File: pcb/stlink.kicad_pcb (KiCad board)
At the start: 4 copper layers, 36.5 x 20 mm, 41 parts, among them J1 USB_A, Q1 S9013, U1 XC6206P332MR, U2 GD32F103CBT6, Y1 8MHz

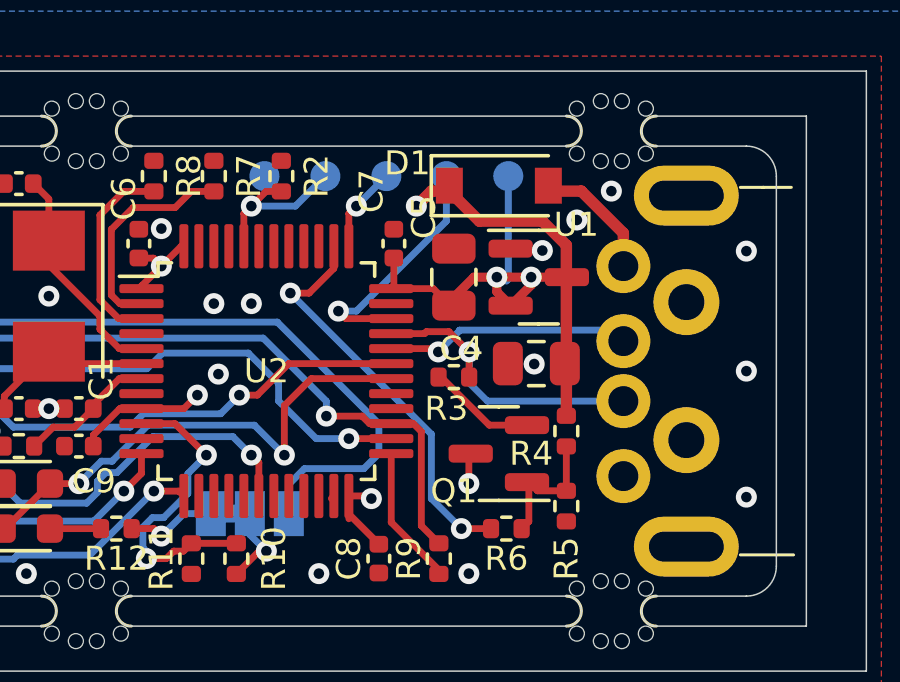
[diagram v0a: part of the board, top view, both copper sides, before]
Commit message: Hmmmm
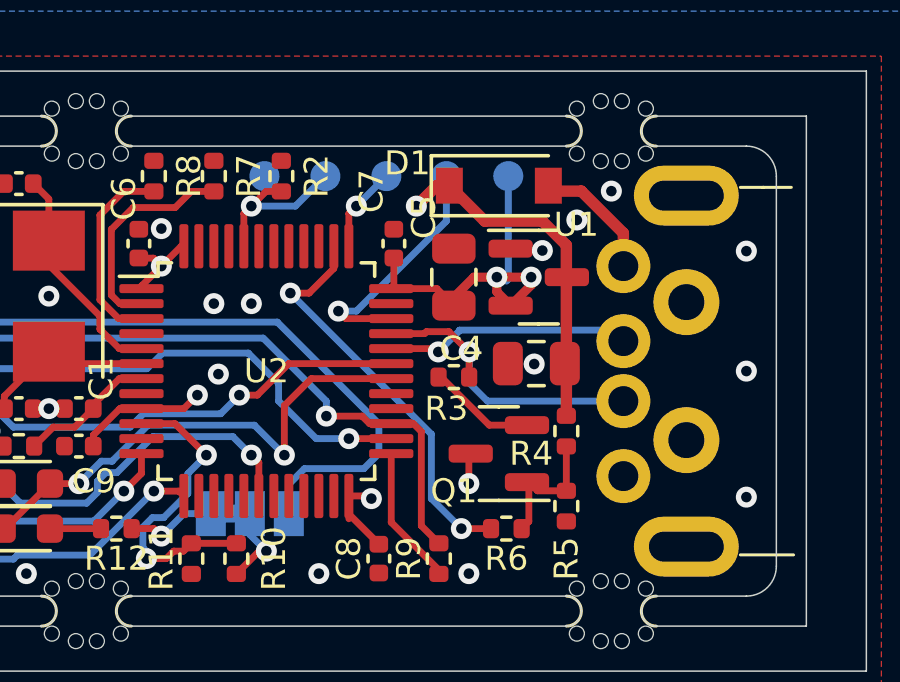
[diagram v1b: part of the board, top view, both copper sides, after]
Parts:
- U2: value GD32F103CBT6 -> STM32F103C8
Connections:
- C5 pad 1: +5V -> +3V3
- C7 pad 1: +5V -> +3V3
- TP1 pad 1: +5V -> +3V3
- U1 pad 2: +5V -> +3V3
- U2 pad 36: +5V -> +3V3
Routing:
- net +5V: track 45.6 -> 32.1 mm, vias 4 -> 2
- net +3V3: track 18.7 -> 30.8 mm, vias 8 -> 10
